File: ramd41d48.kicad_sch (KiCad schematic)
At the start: 14 parts, among them U23 SN74ALS253N (КР1533КП12), U24 SN74ALS253N (КР1533КП12), U26 SN74ALS253N (КР1533КП12), U27 SN74ALS253N (КР1533КП12), U41 2118 (КР565РУ6), U42 2118 (КР565РУ6), U43 2118 (КР565РУ6), U44 2118 (КР565РУ6), U45 2118 (КР565РУ6), U46 2118 (КР565РУ6), U47 2118 (КР565РУ6), U48 2118 (КР565РУ6)

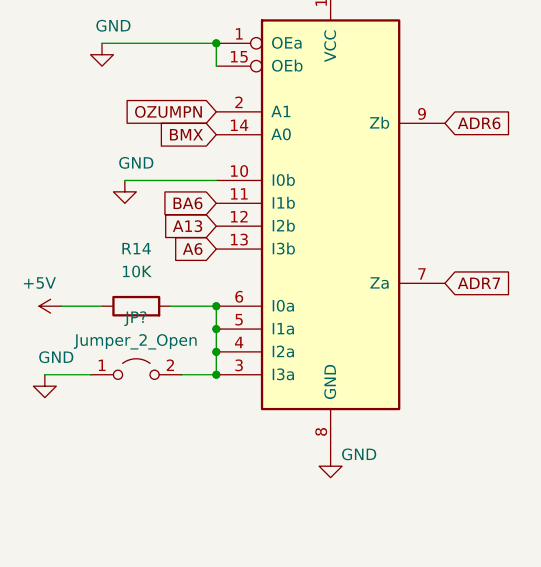
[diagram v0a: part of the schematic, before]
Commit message: March 22nd - 3rd edition
List 3 is complete
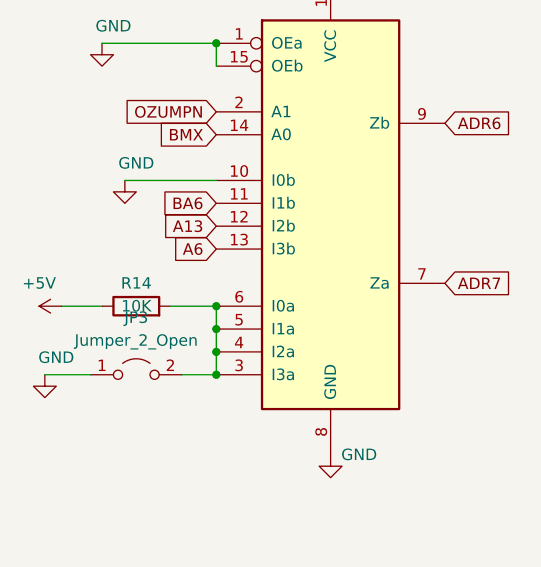
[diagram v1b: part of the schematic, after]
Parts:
- gave numbers to parts that had none: 1
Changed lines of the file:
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@@
   (symbol (lib_id "Jumper:Jumper_2_Open") (at 38.1 134.62 0) (unit 1)
     (in_bom yes) (on_board yes) (fields_autoplaced)
-    (property "Reference" "JP?" (id 0) (at 38.1 128.27 0))
+    (property "Reference" "JP3" (id 0) (at 38.1 128.27 0))
     (property "Value" "Jumper_2_Open" (id 1) (at 38.1 130.81 0))
     (property "Footprint" "Connector_PinHeader_2.54mm:PinHeader_1x02_P2.54mm_Vertical" (id 2) (at 38.1 134.62 0)
@@
   )
   (symbol (lib_id "Device:R") (at 38.1 127 90) (unit 1)
-    (in_bom yes) (on_board yes) (fields_autoplaced)
-    (property "Reference" "R14" (id 0) (at 38.1 120.65 90))
-    (property "Value" "10K" (id 1) (at 38.1 123.19 90))
+    (in_bom yes) (on_board yes)
+    (property "Reference" "R14" (id 0) (at 38.1 124.46 90))
+    (property "Value" "10K" (id 1) (at 38.1 127 90))
     (property "Footprint" "" (id 2) (at 38.1 128.778 90)
       (effects (font (size 1.27 1.27)) hide)
